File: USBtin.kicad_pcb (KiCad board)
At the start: 2 copper layers, 65 x 32 mm, 21 parts, among them IC1 MCP2515-I_P, J1 USB_B, J2 Conn_01x03, U1 PIC18F14K50-EP, U2 MCP2551-I-P, Y1 24MHz

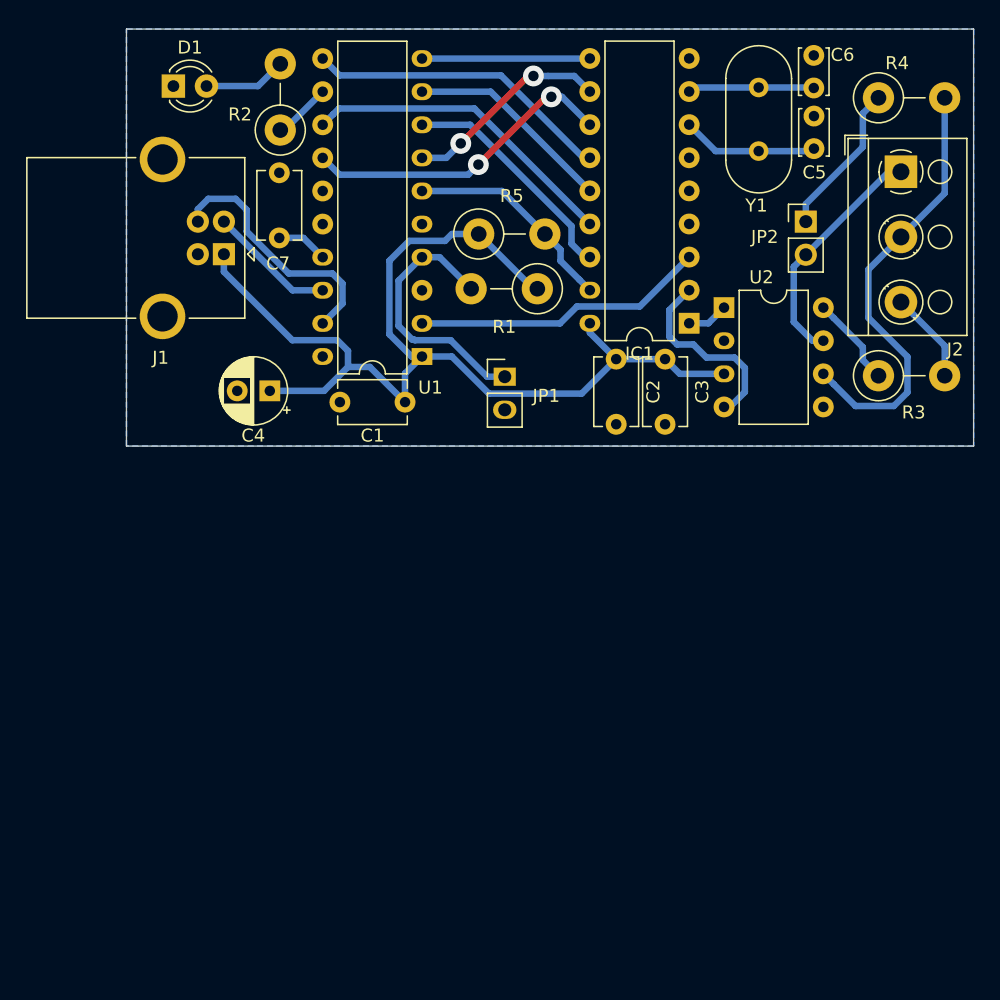
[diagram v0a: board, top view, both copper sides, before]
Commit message: rotate 90 degrees
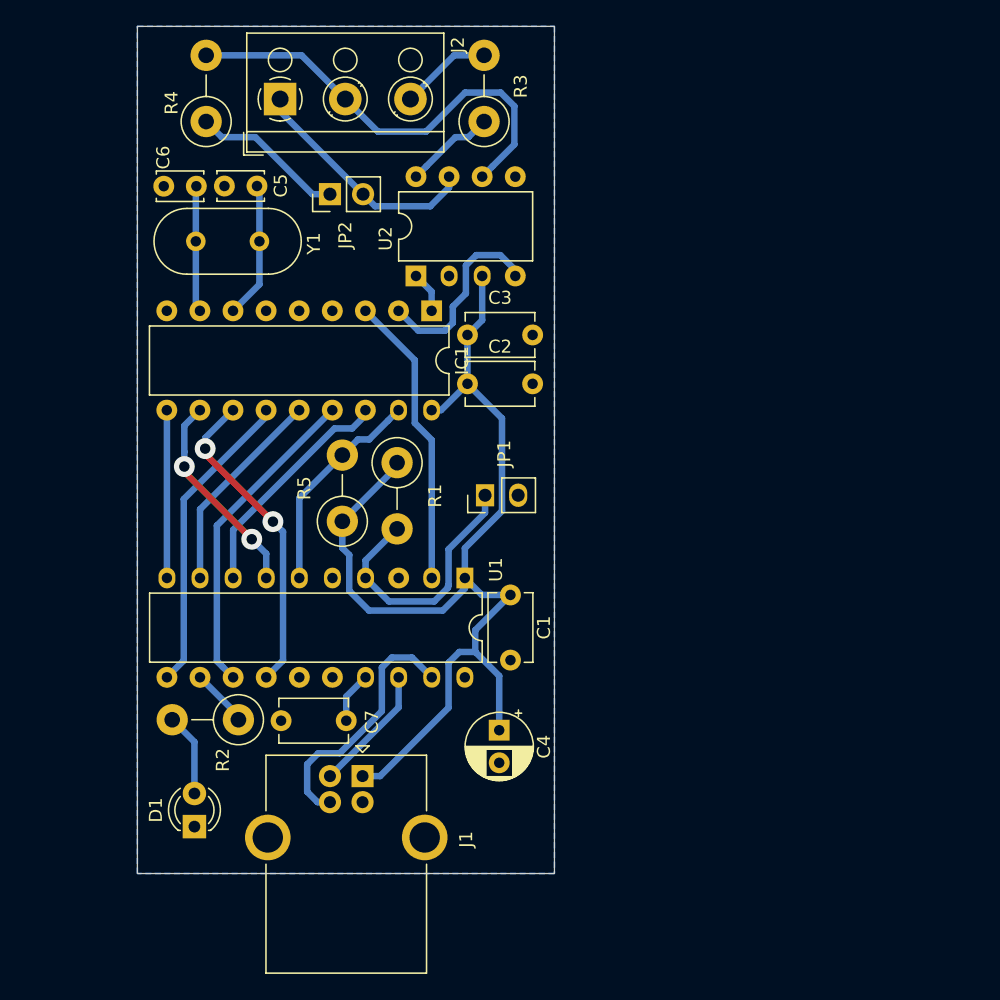
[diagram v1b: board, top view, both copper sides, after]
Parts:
- moved D1 56.8 mm to (105.2, 161.2), turned to 90 degrees
- moved R4 51.6 mm to (106.1, 107.1), turned to 90 degrees
- moved C6 48.0 mm to (105.4, 112.1), turned to 180 degrees
- moved J2 48.0 mm to (111.8, 105.4), turned to 0 degrees
- moved R2 45.4 mm to (108.6, 153.0), turned to 180 degrees
- moved C5 42.8 mm to (110.0, 112.0), turned to 180 degrees
- moved J1 41.4 mm to (118.1, 157.3), turned to 270 degrees
- moved Y1 38.9 mm to (110.2, 116.3), turned to 180 degrees
- moved C7 37.4 mm to (116.9, 153.1), turned to 180 degrees
- moved JP2 36.6 mm to (115.6, 112.7), turned to 90 degrees
- moved R3 36.0 mm to (127.4, 107.1), turned to 90 degrees
- moved C4 31.4 mm to (128.6, 153.8), turned to 270 degrees
- moved R5 24.4 mm to (116.6, 137.8), turned to 90 degrees
- moved U2 23.8 mm to (122.2, 118.9), turned to 90 degrees
- moved IC1 19.8 mm to (123.4, 121.6), turned to 270 degrees
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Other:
- board size 65 x 32 mm -> 32 x 65 mm
